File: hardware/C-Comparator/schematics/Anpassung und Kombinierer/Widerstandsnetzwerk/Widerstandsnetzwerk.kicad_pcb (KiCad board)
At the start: 2 copper layers, 1 part, among them J1 Conn_Coaxial

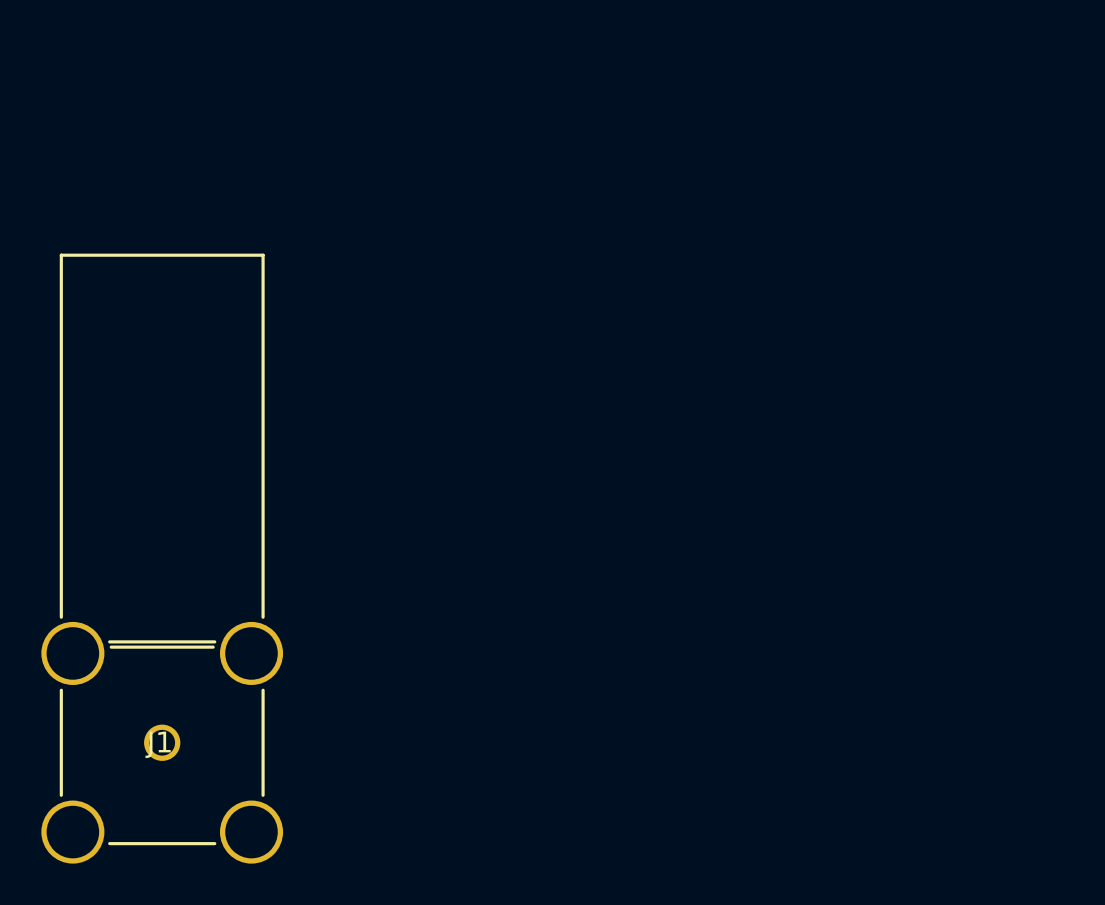
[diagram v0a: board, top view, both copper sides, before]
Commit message: commit on mac
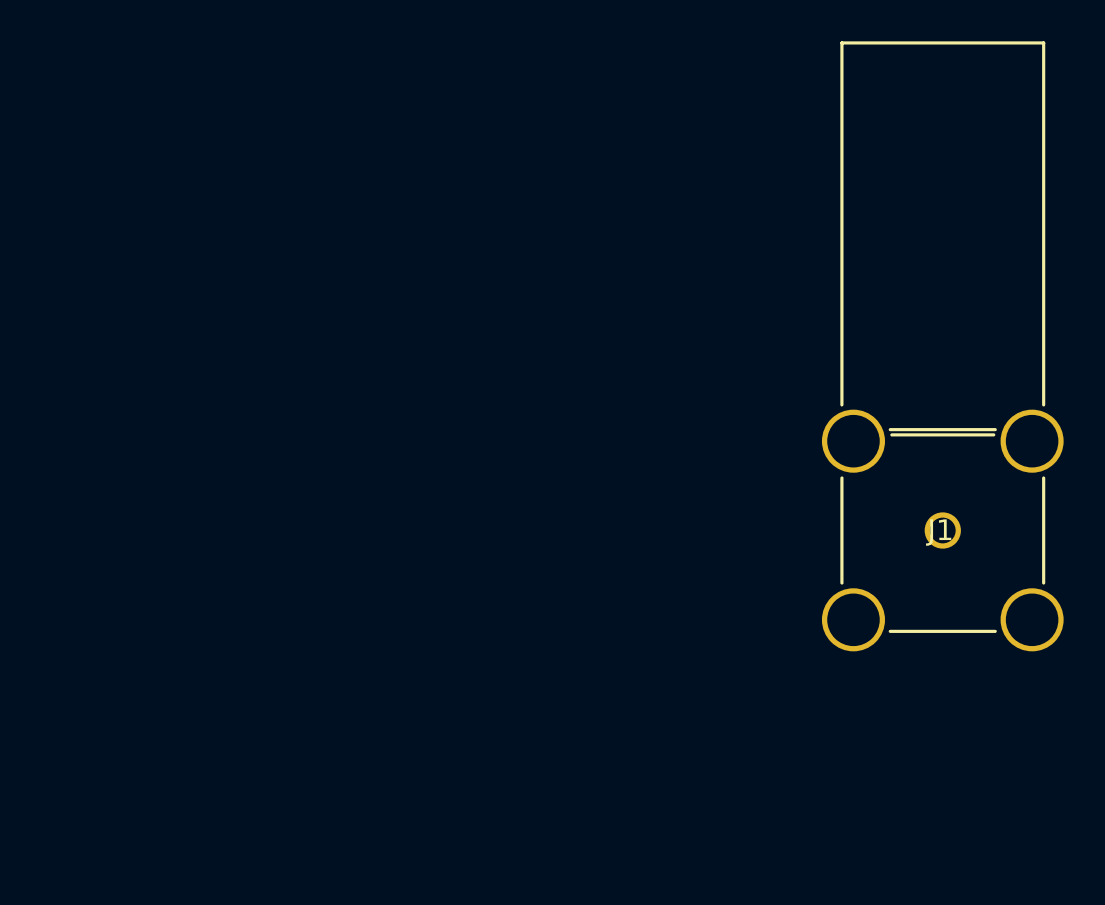
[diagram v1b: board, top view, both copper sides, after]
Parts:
- moved J1 39.1 mm to (102.0, 54.0)
